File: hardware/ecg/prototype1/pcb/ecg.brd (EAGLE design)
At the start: 100 x 80 mm, 21 parts

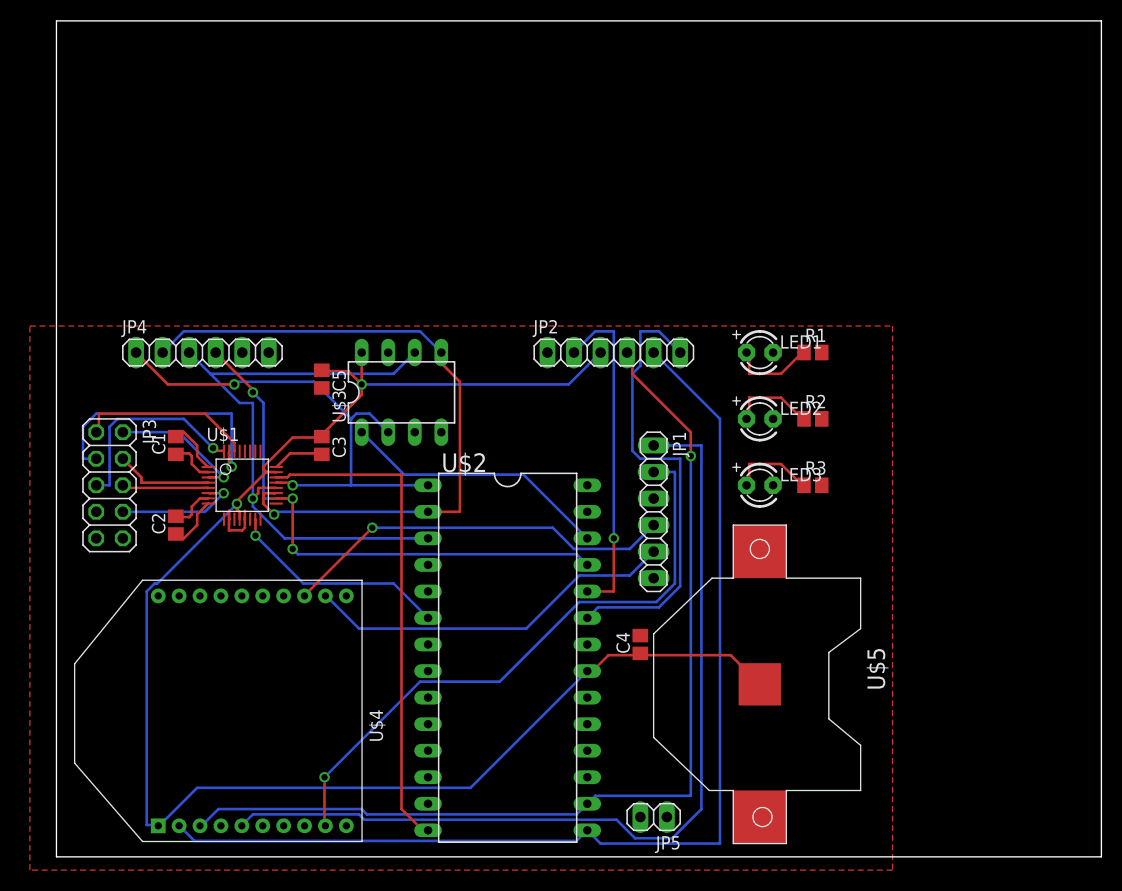
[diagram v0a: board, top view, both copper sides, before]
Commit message: no comment
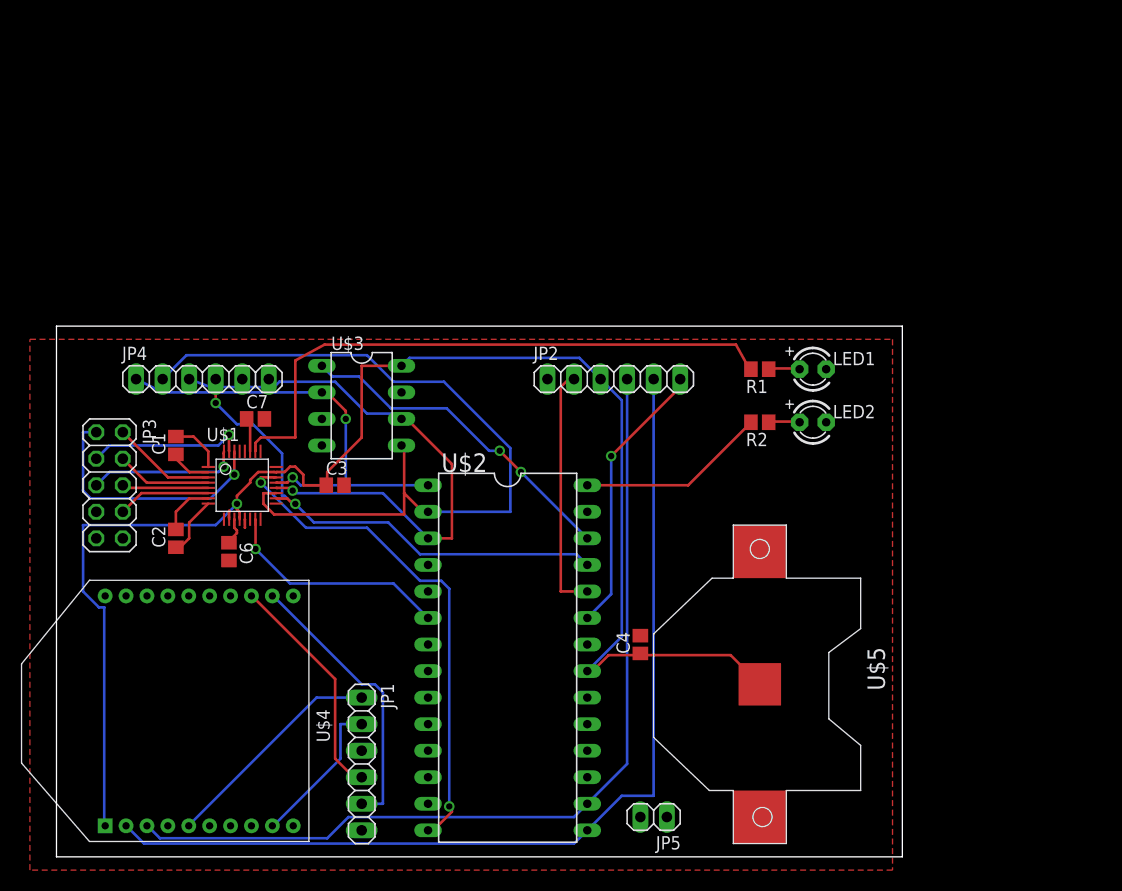
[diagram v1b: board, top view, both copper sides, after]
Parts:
- removed C5: 10uF, adafruit:C0805
- removed LED3: (no value), adafruit:LED3MM
- removed R3: (no value), resistor:R0805
- added C6, C7: 1uF, adafruit:C0805
- moved JP1 36.9 mm to (29.2, 8.89)
- moved LED1 5.32 mm to (72.4, 46.7)
- moved R1 5.32 mm to (67.3, 46.7), turned to 180 degrees
- moved LED2 5.09 mm to (72.4, 41.6)
- moved R2 5.09 mm to (67.3, 41.6), turned to 180 degrees
- moved U$4 5.08 mm to (10.2, 14.0)
- moved U$3 4.02 mm to (29.2, 43.2), turned to 270 degrees
- moved C3 4.02 mm to (26.7, 35.6), turned to 0 degrees
- moved JP2 2.54 mm to (53.3, 45.7)
- moved JP4 2.54 mm to (14.0, 45.7)
- moved C2 1.27 mm to (11.4, 30.5)
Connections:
- removed net N$28: C3.2, U$1.P$24
- removed net N$31: LED3.A, R3.1
- new net N$27: C6.1, U$1.P$11
- new net N$32: C7.1, U$1.P$27
- new net ULED1: R1.2, U$1.P$26
- new net ULED2: R2.2, U$2.28
- net GND: now also C3.2, C6.2, C7.2, U$1.P$24; no longer C5.2, LED3.K
- net VDD: now also JP5.1; no longer C5.1
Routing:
- net N$18: track 85.9 -> 21.6 mm
- net ULED1: track 0.00 -> 57.6 mm
- net N$19: track 58.6 -> 14.5 mm, vias 1 -> 0
- net ULED2: track 0.00 -> 18.2 mm
- net N$20: track 43.6 -> 26.5 mm, vias 0 -> 1
- net N$25: track 37.9 -> 22.2 mm, vias 1 -> 0
- net N$6: track 65.9 -> 77.7 mm, vias 1 -> 0
- net N$16: track 25.7 -> 15.2 mm
- net N$22: track 102.9 -> 93.0 mm
- net VDD: track 153.6 -> 144.6 mm, vias 2 -> 1
- net N$26: track 35.7 -> 27.1 mm
- net N$31: track 8.22 -> 0.00 mm
- net N$17: track 16.8 -> 24.8 mm, vias 0 -> 1
- net N$24: track 32.1 -> 24.4 mm, vias 1 -> 0
- net N$23: track 93.5 -> 86.2 mm, vias 1 -> 0
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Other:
- board size 100 x 80 mm -> 81 x 50.8 mm
